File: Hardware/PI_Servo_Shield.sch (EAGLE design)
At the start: 52 parts, among them J1 RASPBERRYPI-40-PIN-GPIO_PTH_N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, U1 FT231XS, U2 PCA9306, U3 PCA9685

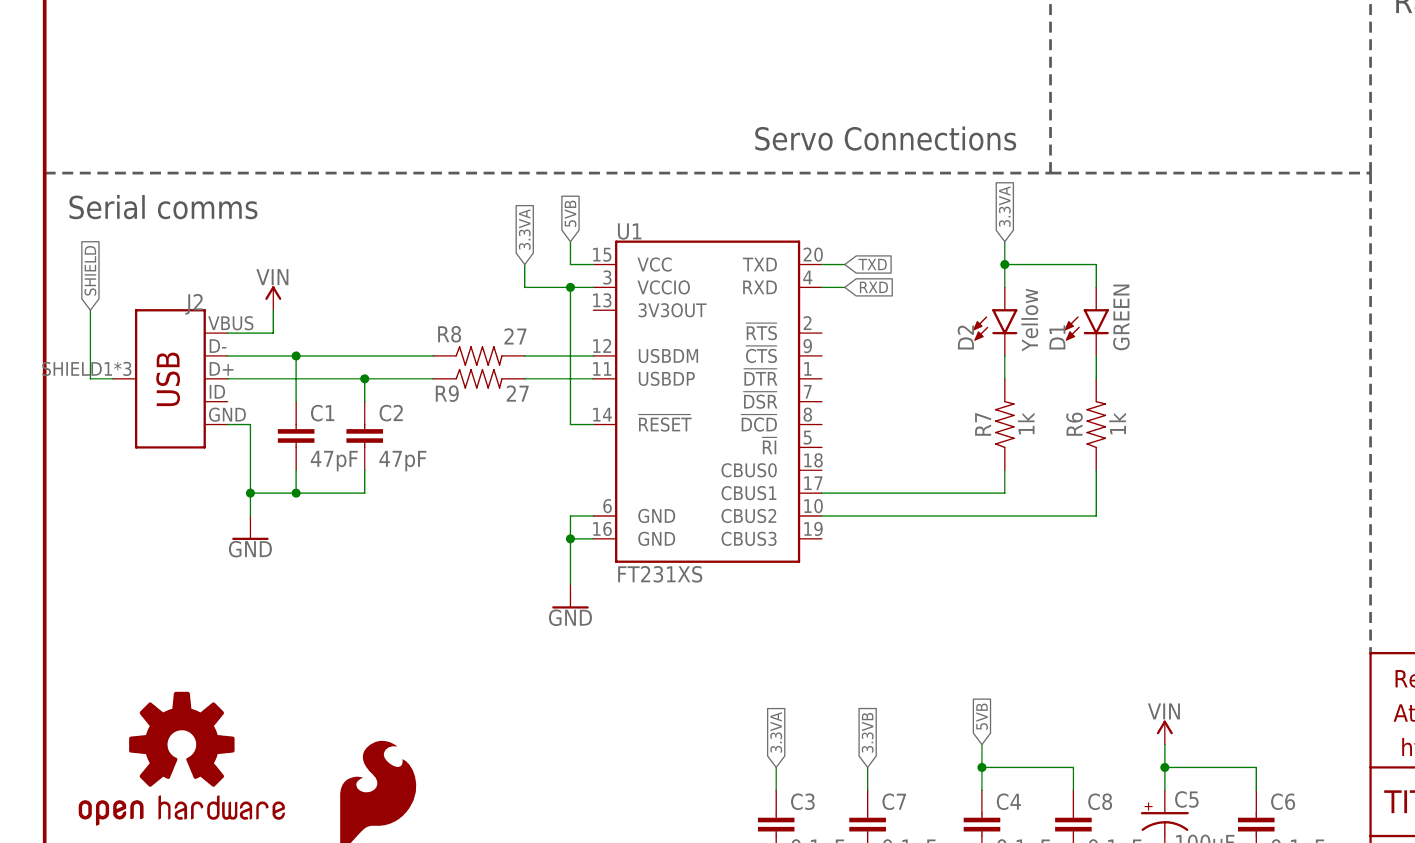
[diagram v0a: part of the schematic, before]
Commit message: Change to v10
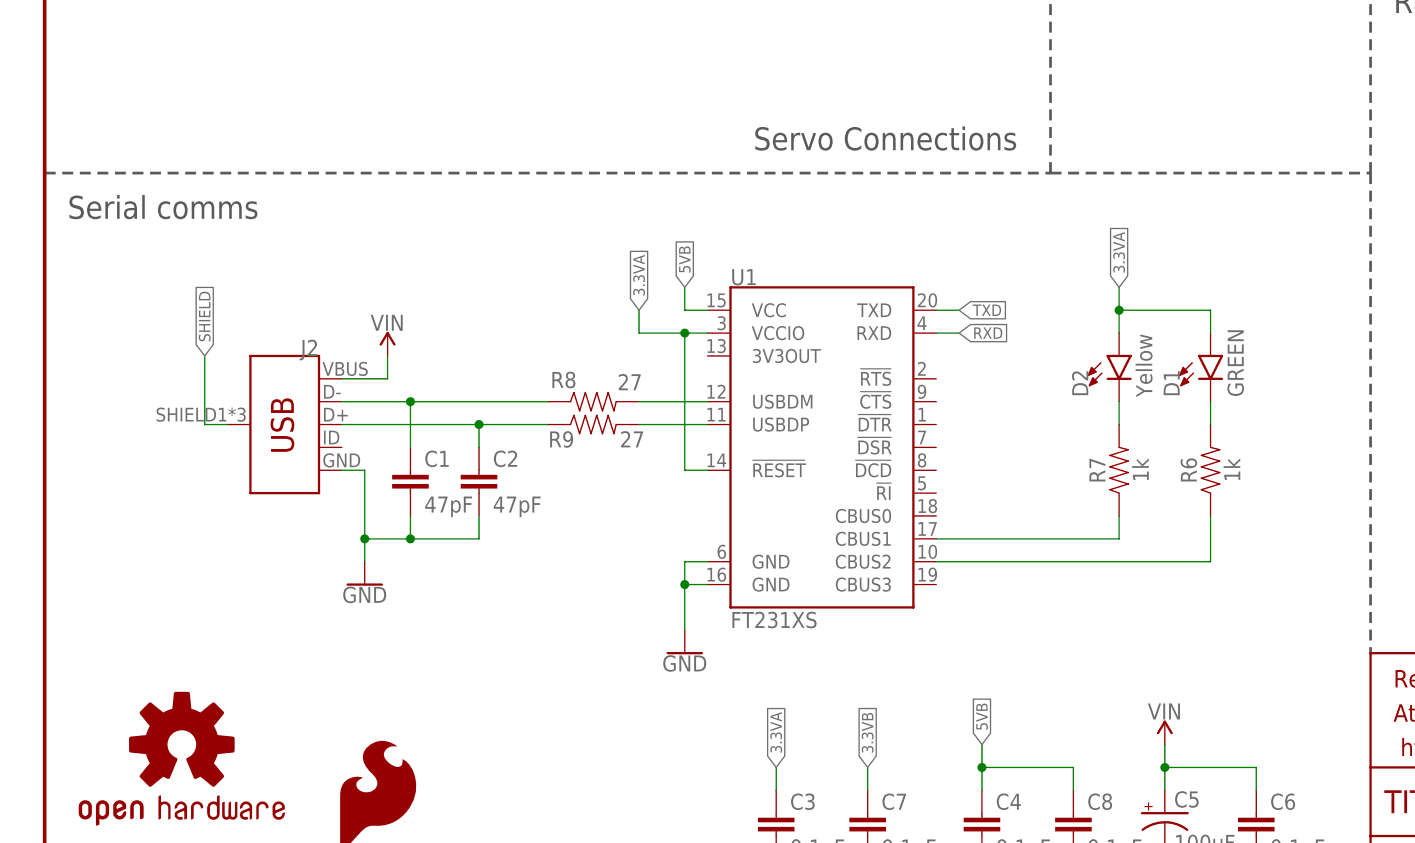
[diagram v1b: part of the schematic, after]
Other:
- moved on the sheet: C1, C2, D1, D2, J2, R6, R7, R8, R9, U1
